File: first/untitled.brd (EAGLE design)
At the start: 160 x 100 mm, 13 parts

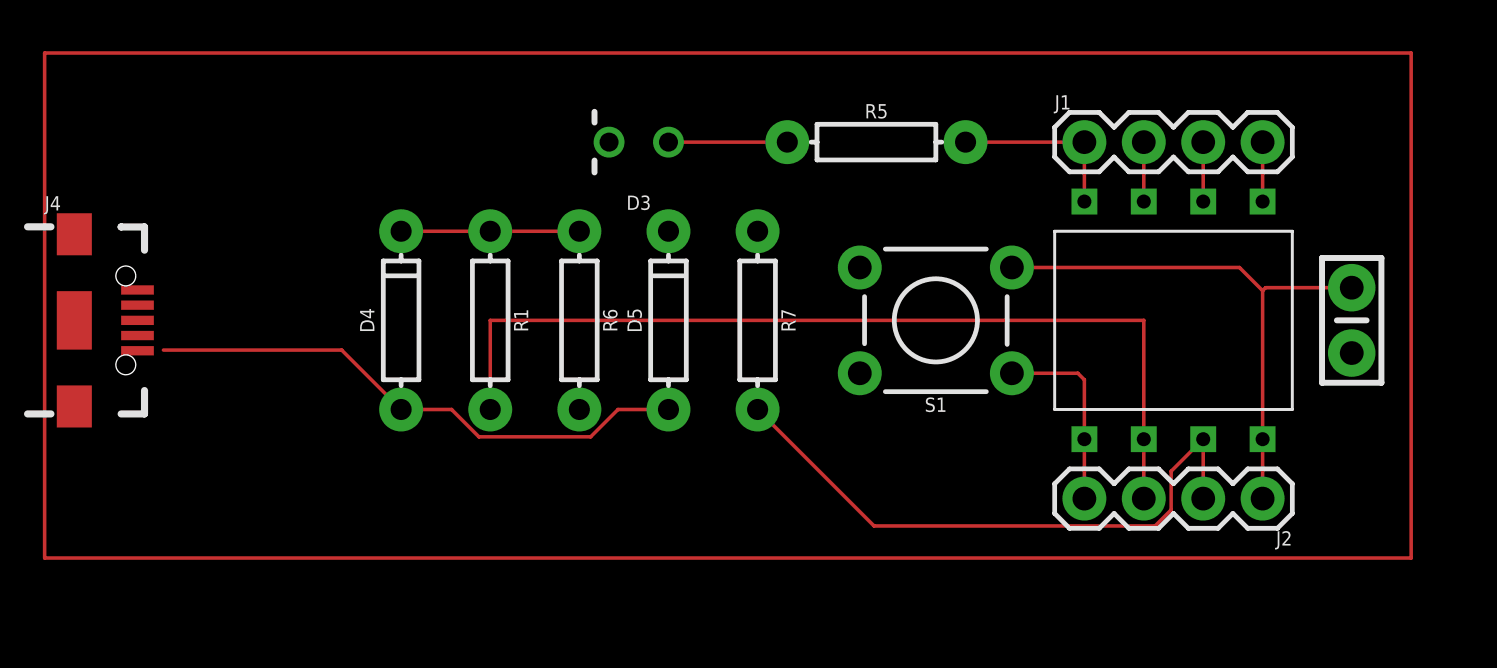
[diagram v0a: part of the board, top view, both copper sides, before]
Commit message: badges
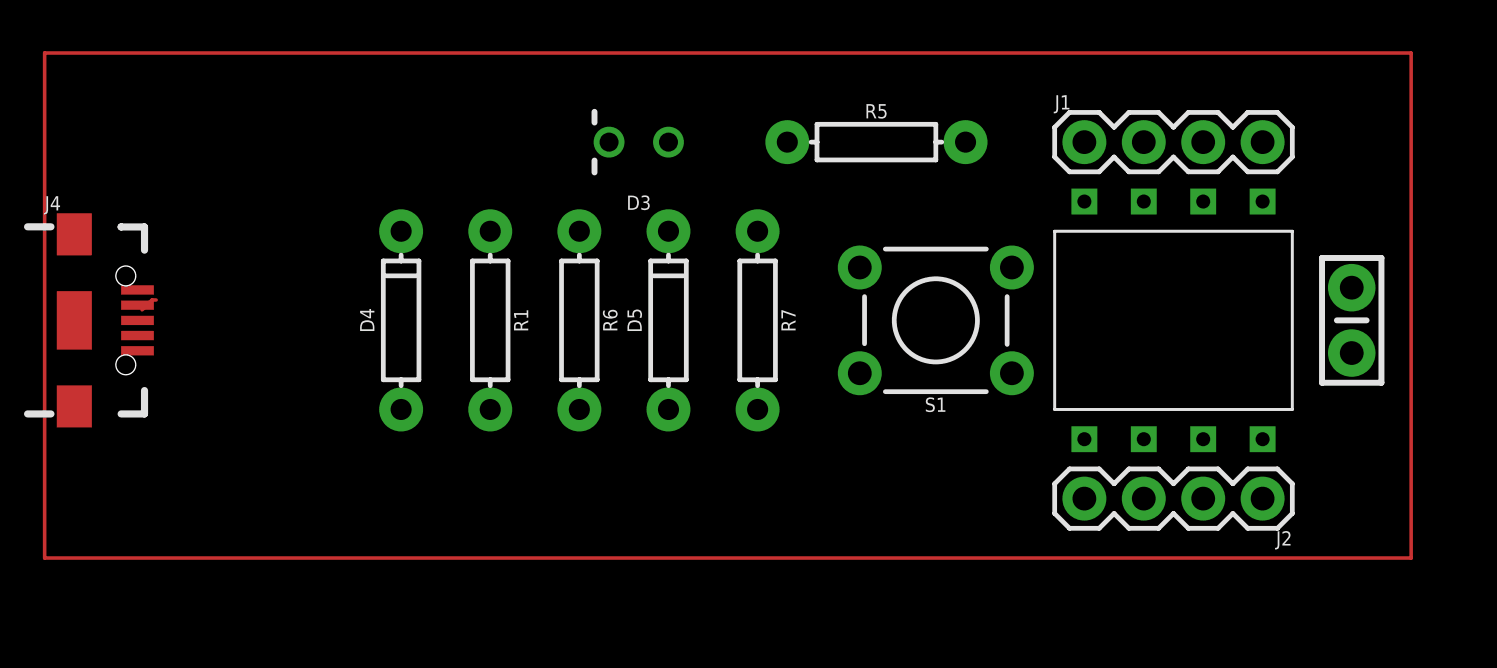
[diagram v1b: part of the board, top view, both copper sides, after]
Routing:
- net GND: track 47.5 -> 0.00 mm
- net PB3: track 39.4 -> 0.00 mm
- net PB4: track 26.2 -> 0.00 mm
- net RESET: track 8.29 -> 0.00 mm
- net N$6: track 7.62 -> 0.00 mm
- net VCC: track 7.62 -> 0.18 mm
- net N$1: track 5.08 -> 0.00 mm
- net PB2: track 2.54 -> 0.00 mm
- net PB1: track 2.54 -> 0.00 mm
- net PB0: track 2.54 -> 0.00 mm
- net N$5: track 0.00 -> 0.77 mm
